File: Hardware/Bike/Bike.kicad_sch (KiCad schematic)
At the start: 18 parts, among them U1 ESP32-WROOM-32

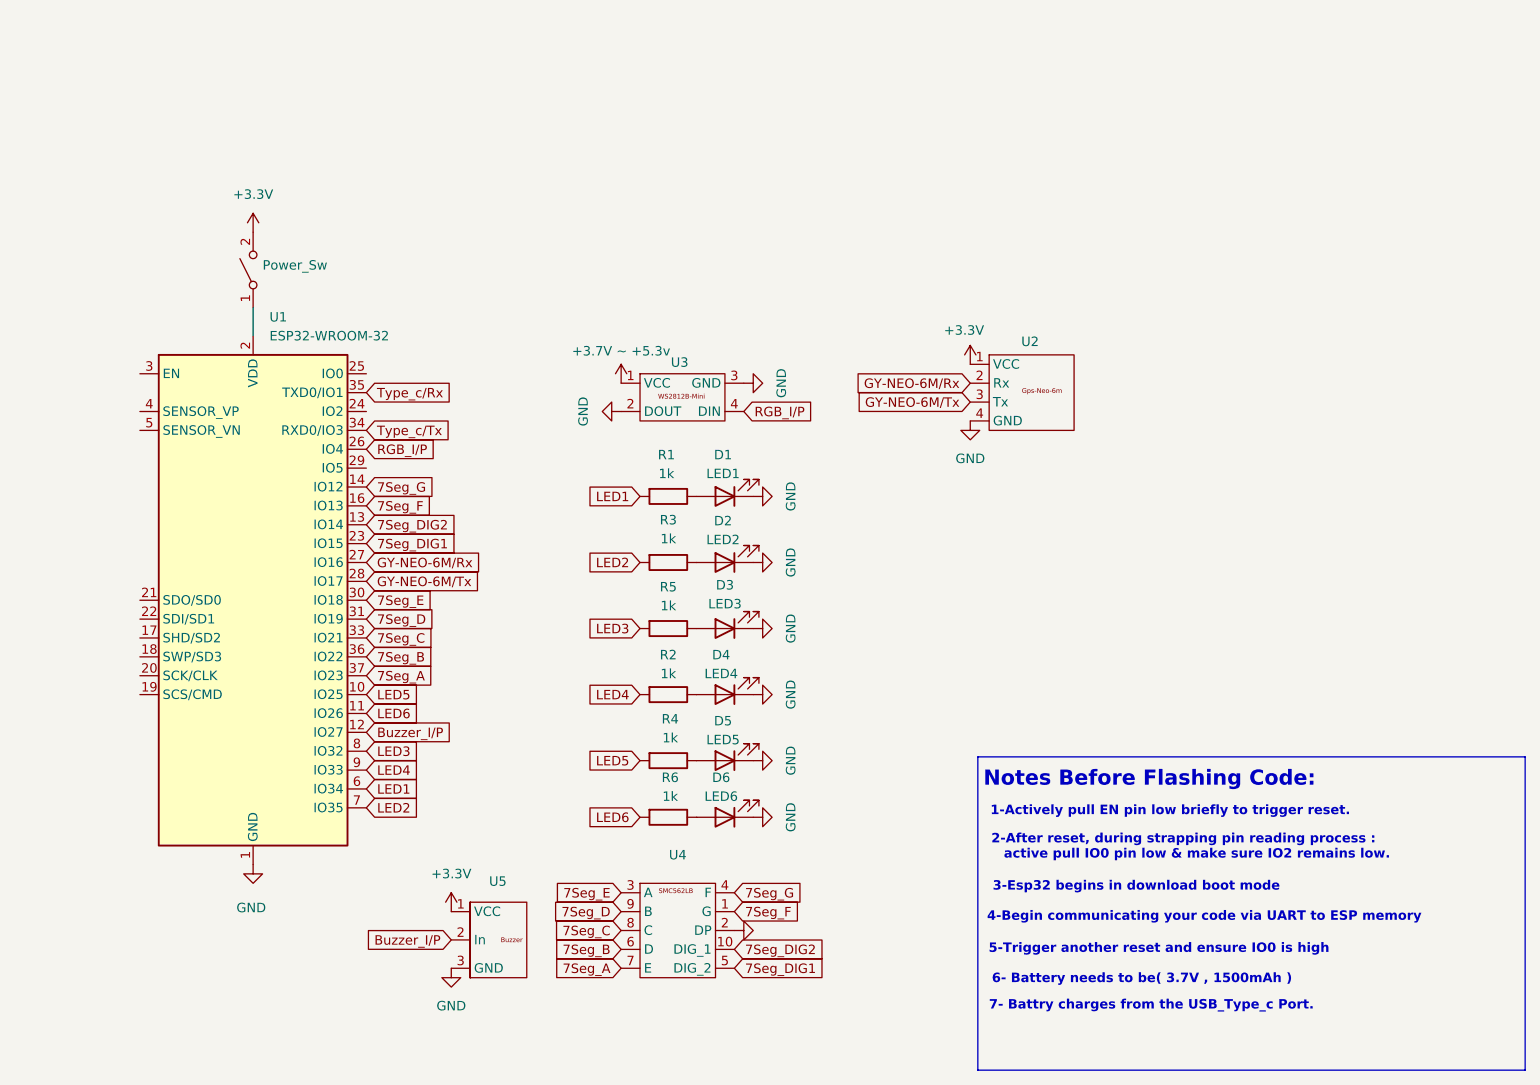
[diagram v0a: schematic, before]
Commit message: Updated Schematic
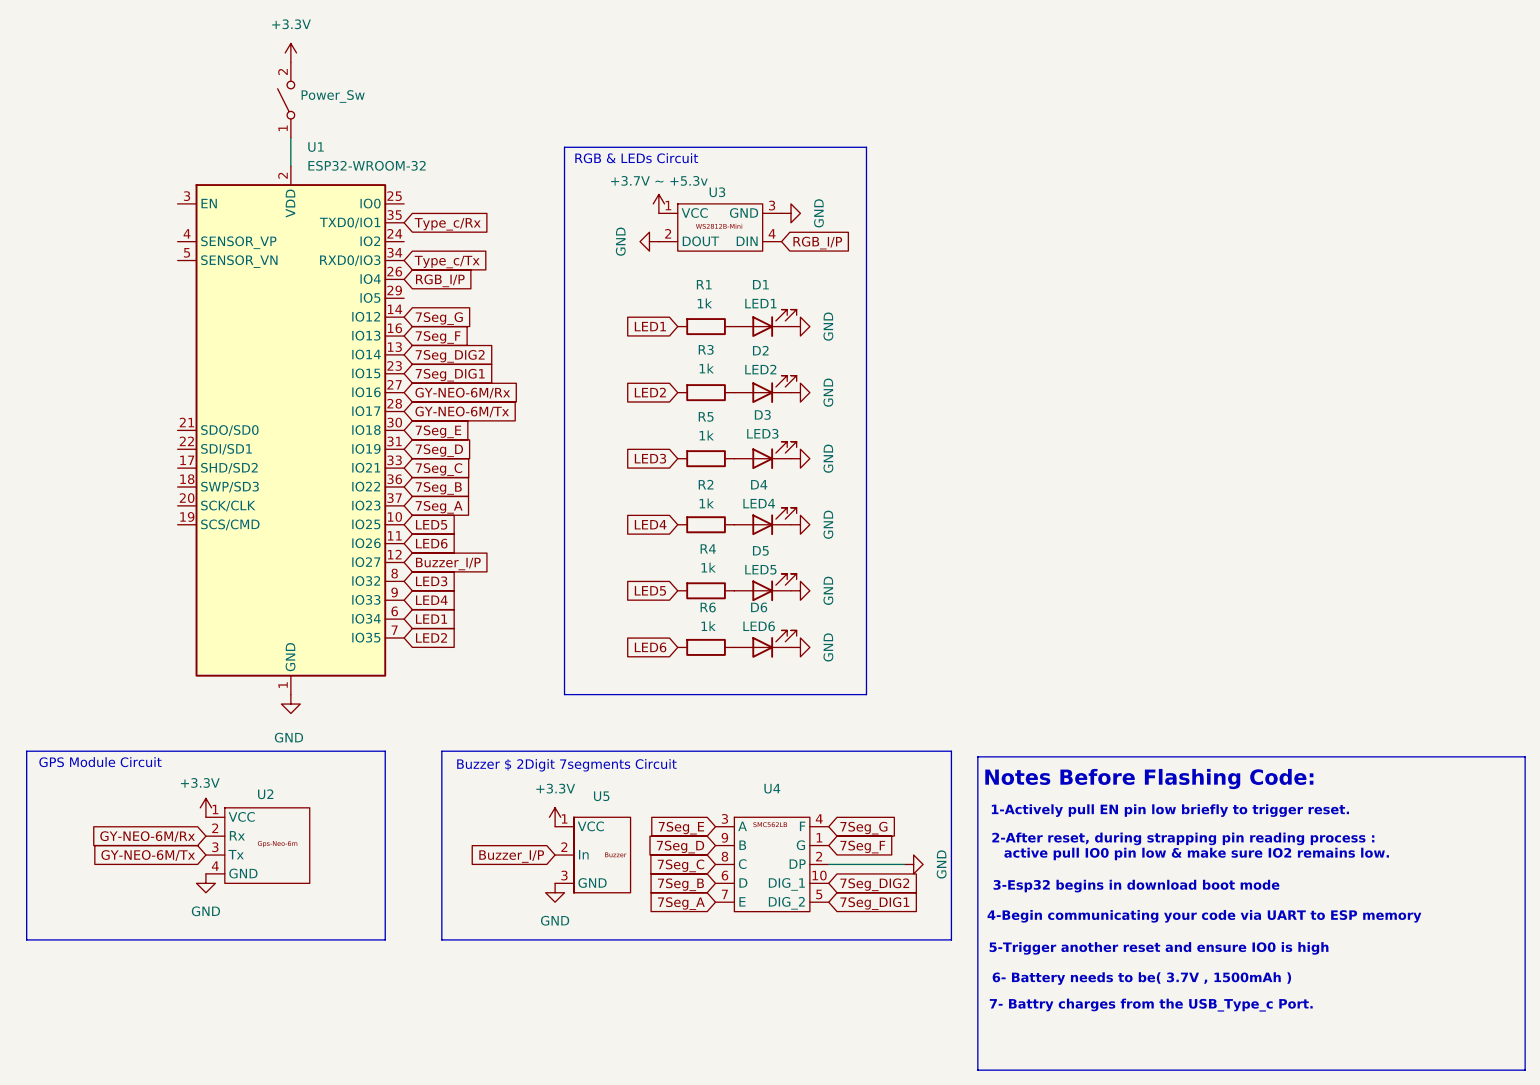
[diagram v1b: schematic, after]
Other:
- note added: "Buzzer $ 2Digit 7segments Circuit"
- note added: "GPS Module Circuit"
- note added: "RGB & LEDs Circuit"
- moved on the sheet: D1, D2, D3, D4, D5, D6, Power_Sw, R1, R2, R3, R4, R5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
